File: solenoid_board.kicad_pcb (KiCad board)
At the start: 2 copper layers, 170 x 145 mm, 68 parts, among them J2 MCU_LEFT_LEGS, J3 MCU_RIGHT_LEGS

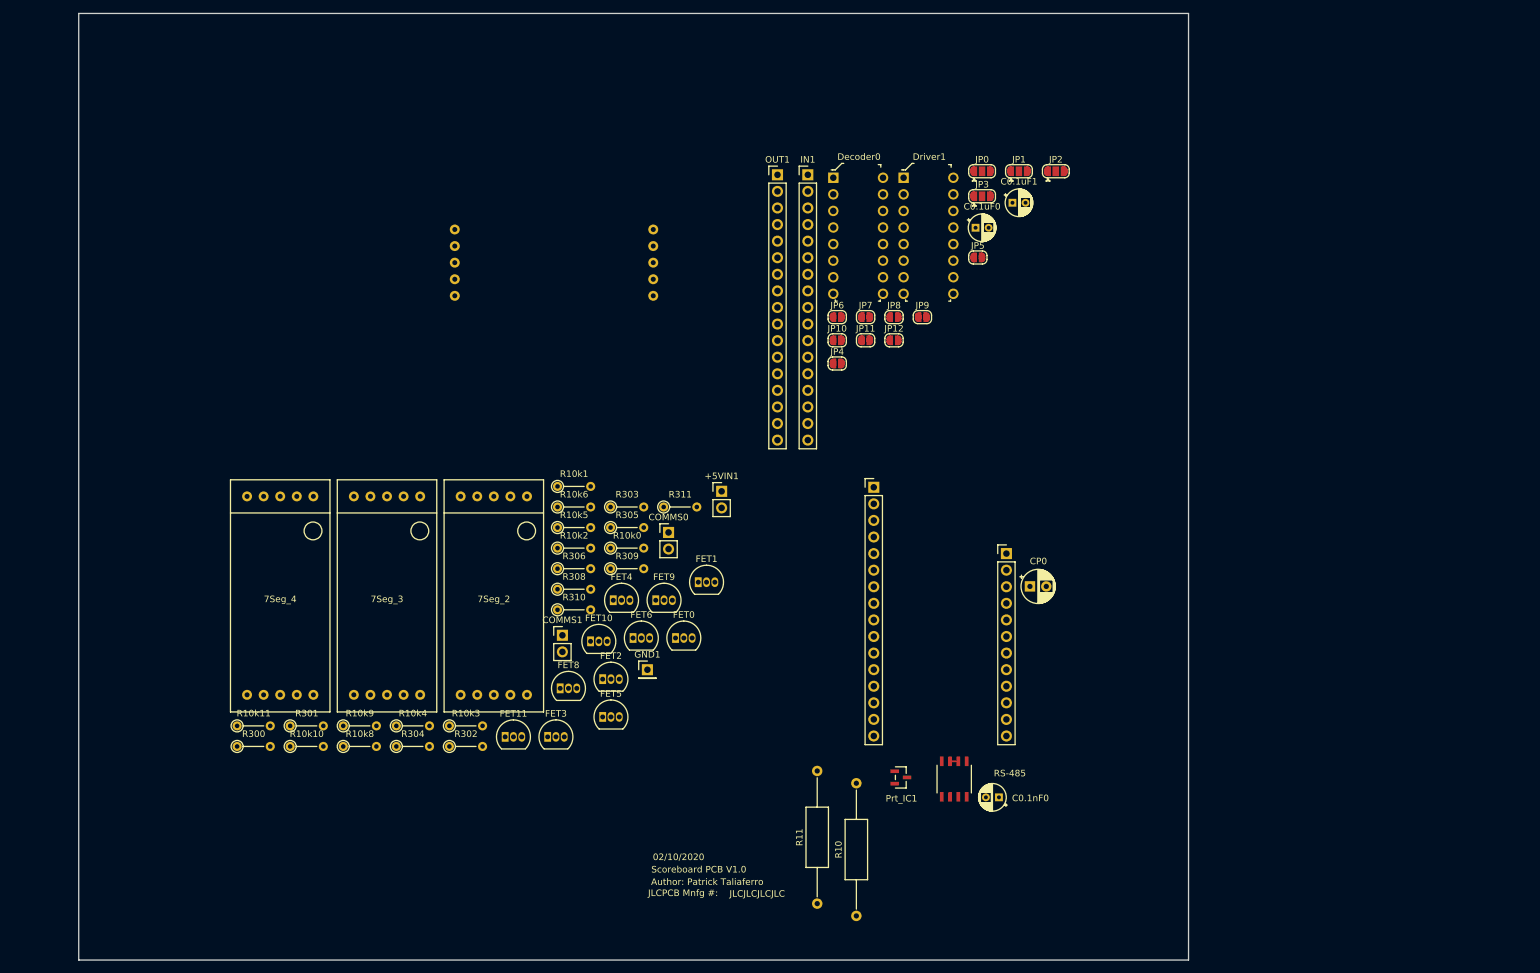
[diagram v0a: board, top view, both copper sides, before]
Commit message: Serious Geometry design occurred.
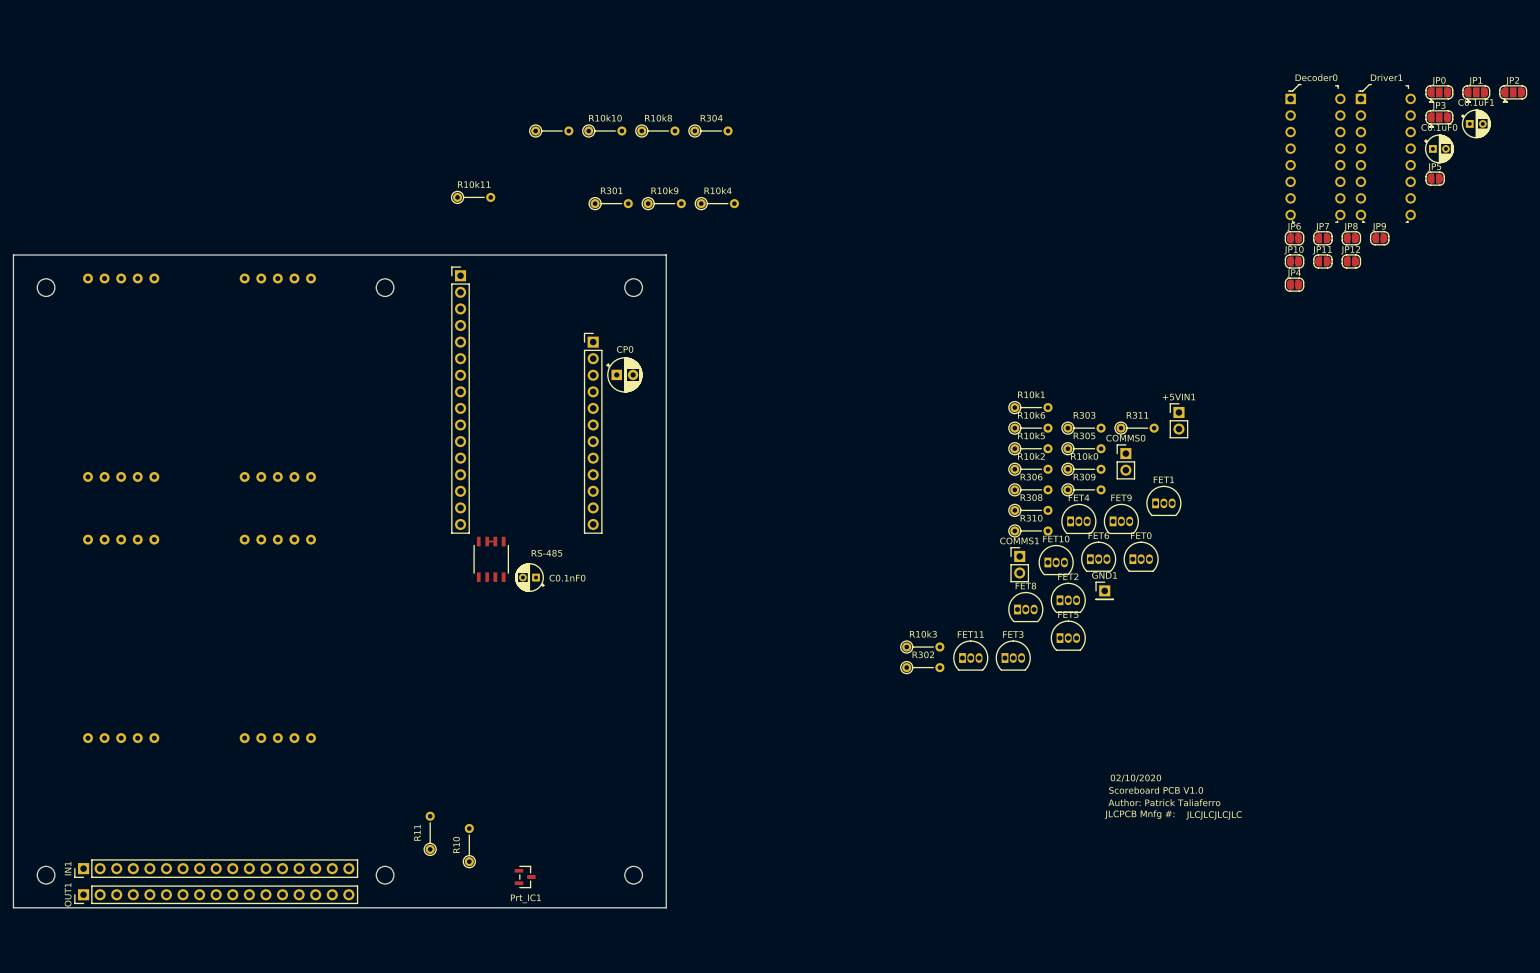
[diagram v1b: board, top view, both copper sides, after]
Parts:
- added REF**: MountingHole_2.7mm_M2.5, MountingHole:MountingHole_2.7mm_M2.5, F.Cu at (140.0, 57.0)
- added REF**: MountingHole_2.7mm_M2.5, MountingHole:MountingHole_2.7mm_M2.5, F.Cu at (140.0, 147.0)
- added REF**: MountingHole_2.7mm_M2.5, MountingHole:MountingHole_2.7mm_M2.5, F.Cu at (101.9, 147.0)
- added REF**: MountingHole_2.7mm_M2.5, MountingHole:MountingHole_2.7mm_M2.5, F.Cu at (101.9, 57.0)
- added REF**: MountingHole_2.7mm_M2.5, MountingHole:MountingHole_2.7mm_M2.5, F.Cu at (50.0, 57.0)
- added REF**: MountingHole_2.7mm_M2.5, MountingHole:MountingHole_2.7mm_M2.5, F.Cu at (50.0, 147.0)
- 7Seg_2, 7Seg_3, 7Seg_4: moved to B.Cu
- R10, R11: footprint Resistor_THT:R_Axial_DIN0309_L9.0mm_D3.2mm_P20.32mm_Horizontal -> Resistor_THT:R_Axial_DIN0204_L3.6mm_D1.6mm_P5.08mm_Vertical
- moved IN1 153.6 mm to (55.7, 146.0), turned to 90 degrees
- moved OUT1 153.2 mm to (55.7, 150.0), turned to 90 degrees
- moved R10k10 104.8 mm to (133.1, 33.0)
- moved R10k8 104.8 mm to (141.3, 33.0)
- moved R300 104.8 mm to (125.0, 33.0)
- moved R304 104.8 mm to (149.4, 33.0)
- moved R10k4 92.6 mm to (150.4, 44.1)
- moved R10k9 92.6 mm to (142.2, 44.1)
- moved R301 92.6 mm to (134.1, 44.1)
- moved R10k11 87.7 mm to (113.0, 43.2)
- moved C0.1nF0 78.5 mm to (125.0, 101.4)
- moved RS-485 78.5 mm to (118.2, 98.6)
- moved 7Seg_1 71.4 mm to (85.5, 110.8), turned to 0 degrees
- moved CP0 71.1 mm to (137.4, 70.4)
- moved J3 71.1 mm to (133.8, 65.3)
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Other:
- board size 170 x 145 mm -> 100 x 100 mm
